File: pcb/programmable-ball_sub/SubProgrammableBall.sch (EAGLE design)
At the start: 9 parts, among them CON1 B4B-ZR-SM4-TF, U2 LSM6DS0TR

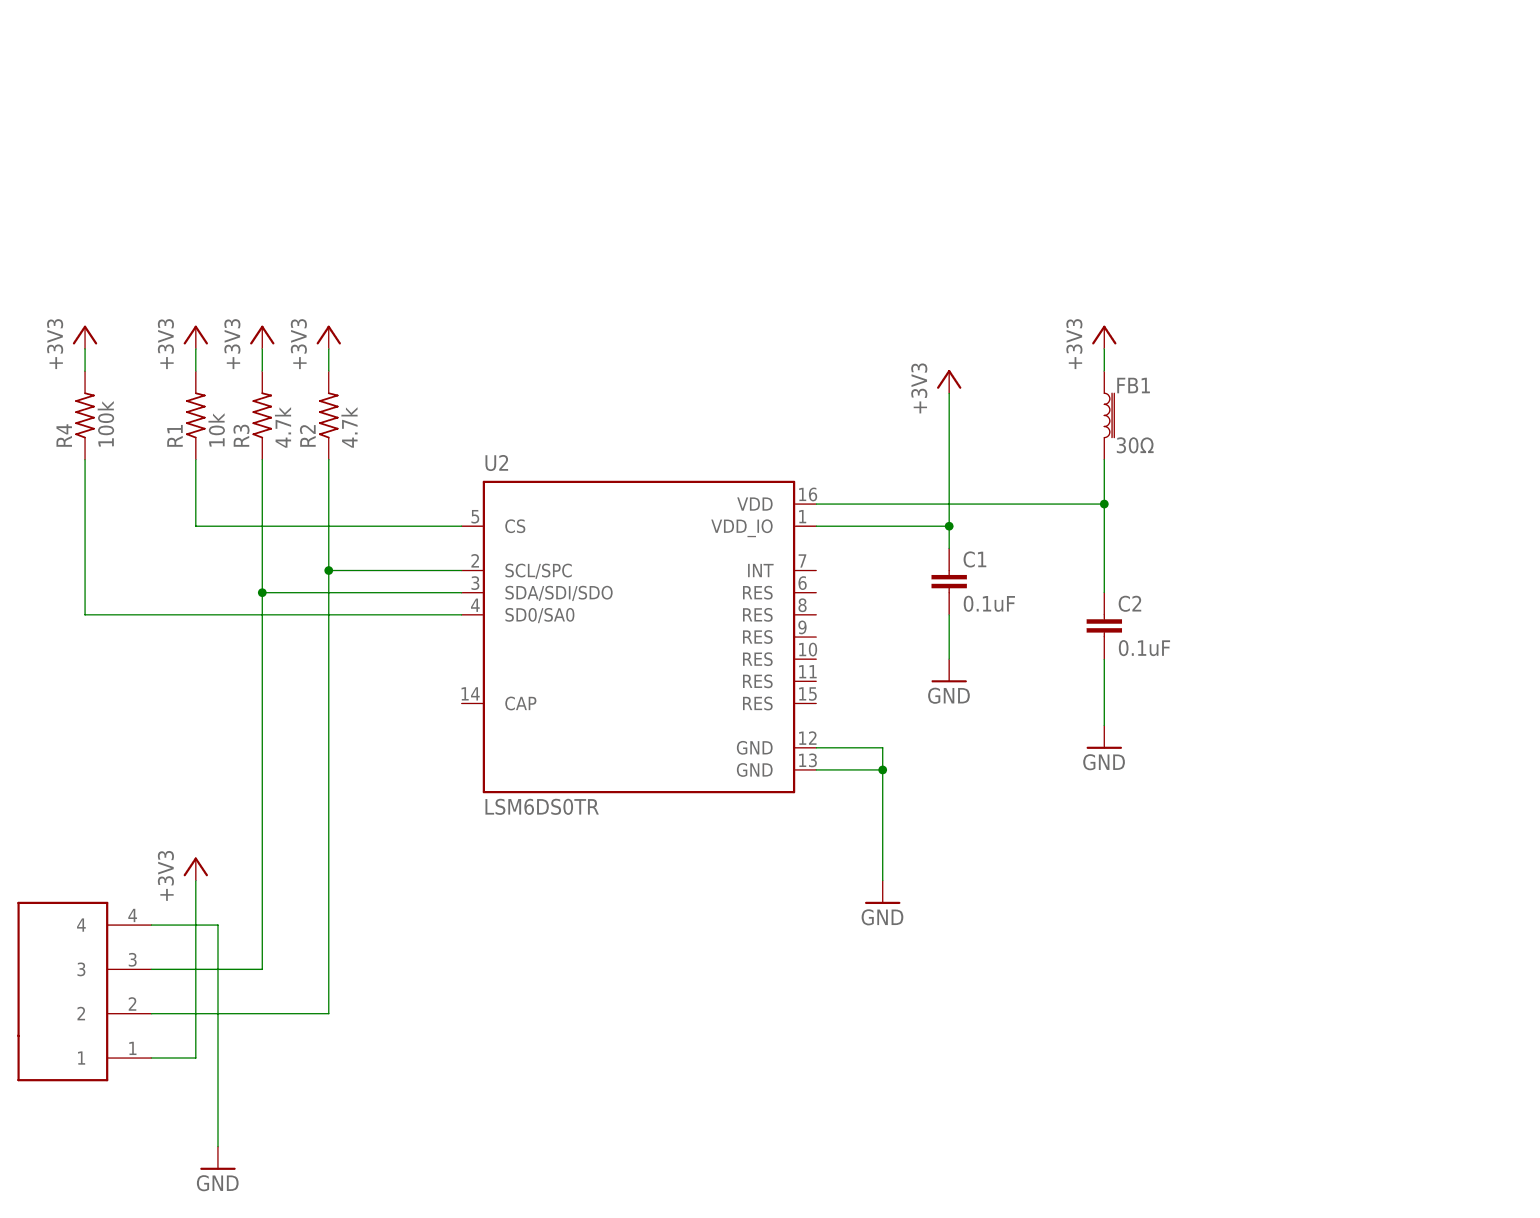
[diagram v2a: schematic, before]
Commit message: 軽微な修正
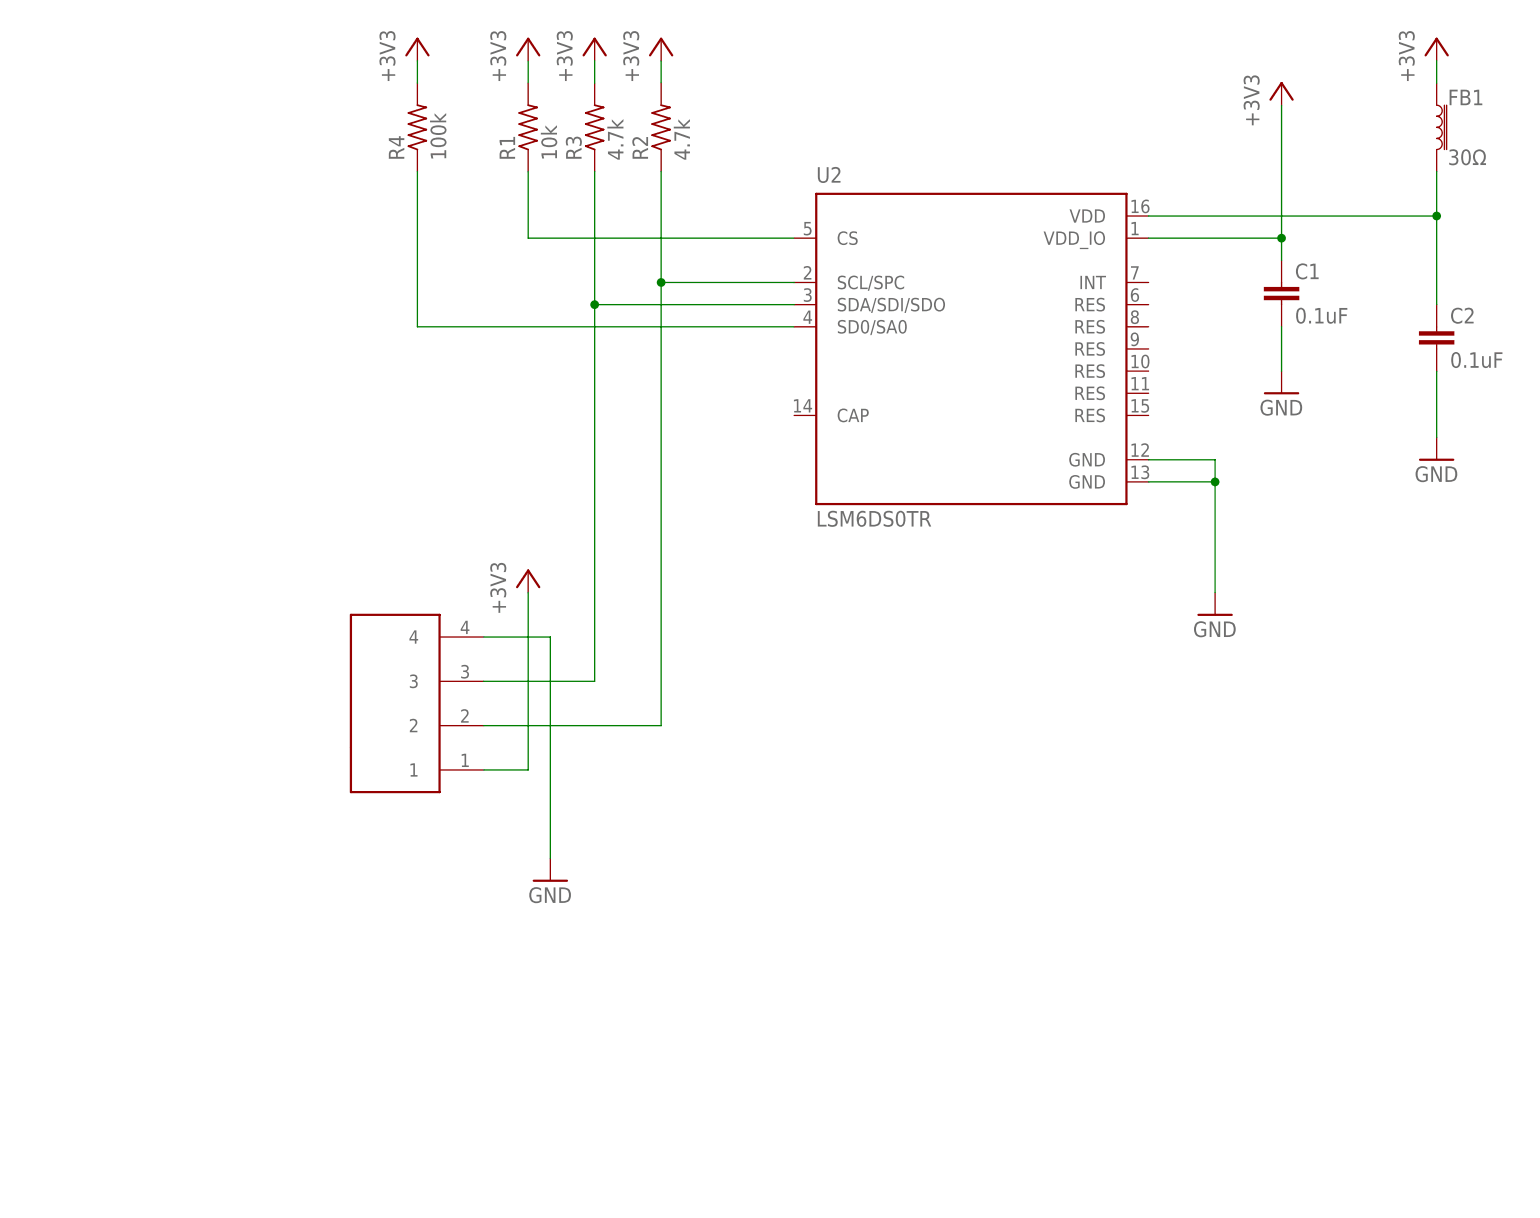
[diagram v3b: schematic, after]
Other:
- moved on the sheet: C1, C2, FB1, R1, R2, R3, R4, U2
